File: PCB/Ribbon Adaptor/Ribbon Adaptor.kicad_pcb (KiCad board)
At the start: 2 copper layers, 20 x 24.5 mm, 6 parts, among them J1 10056847-101LF, J2 AFC07-S20FCC-00

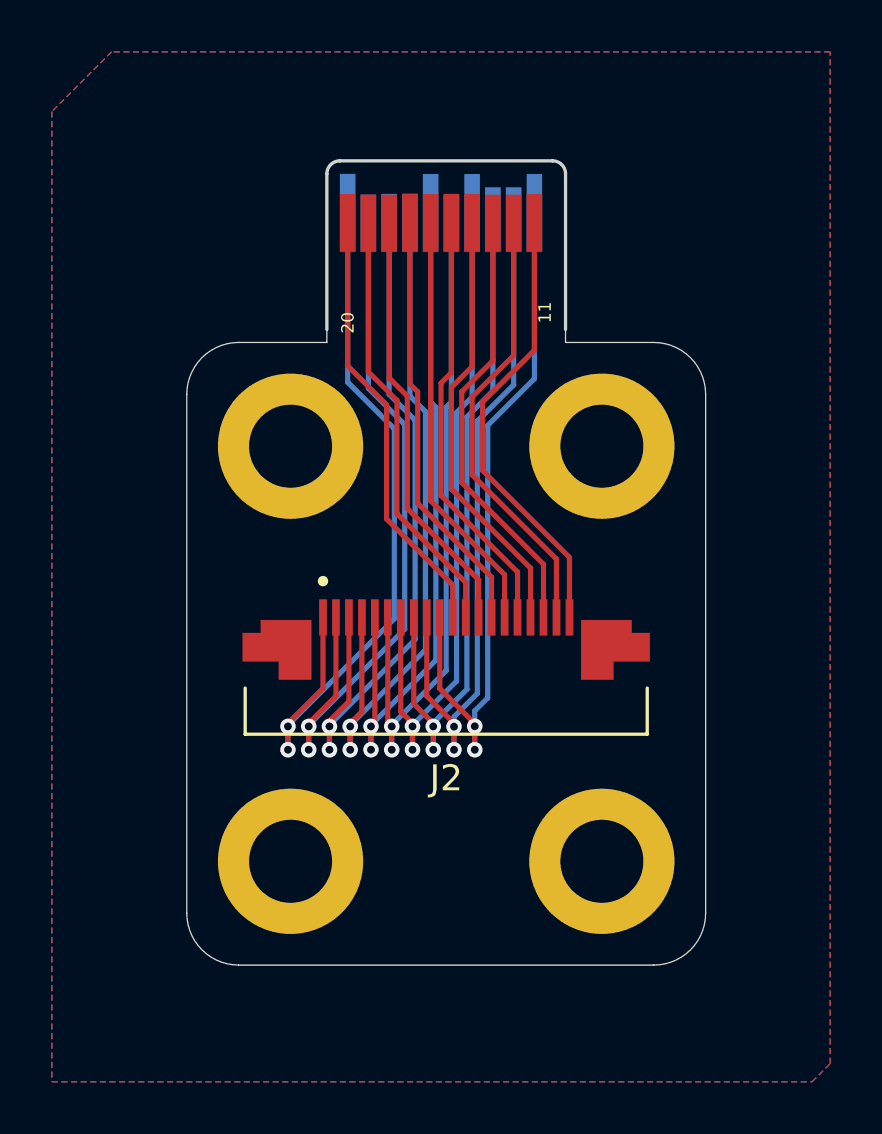
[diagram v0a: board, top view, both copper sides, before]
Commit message: Started code, commiting before adding submodules
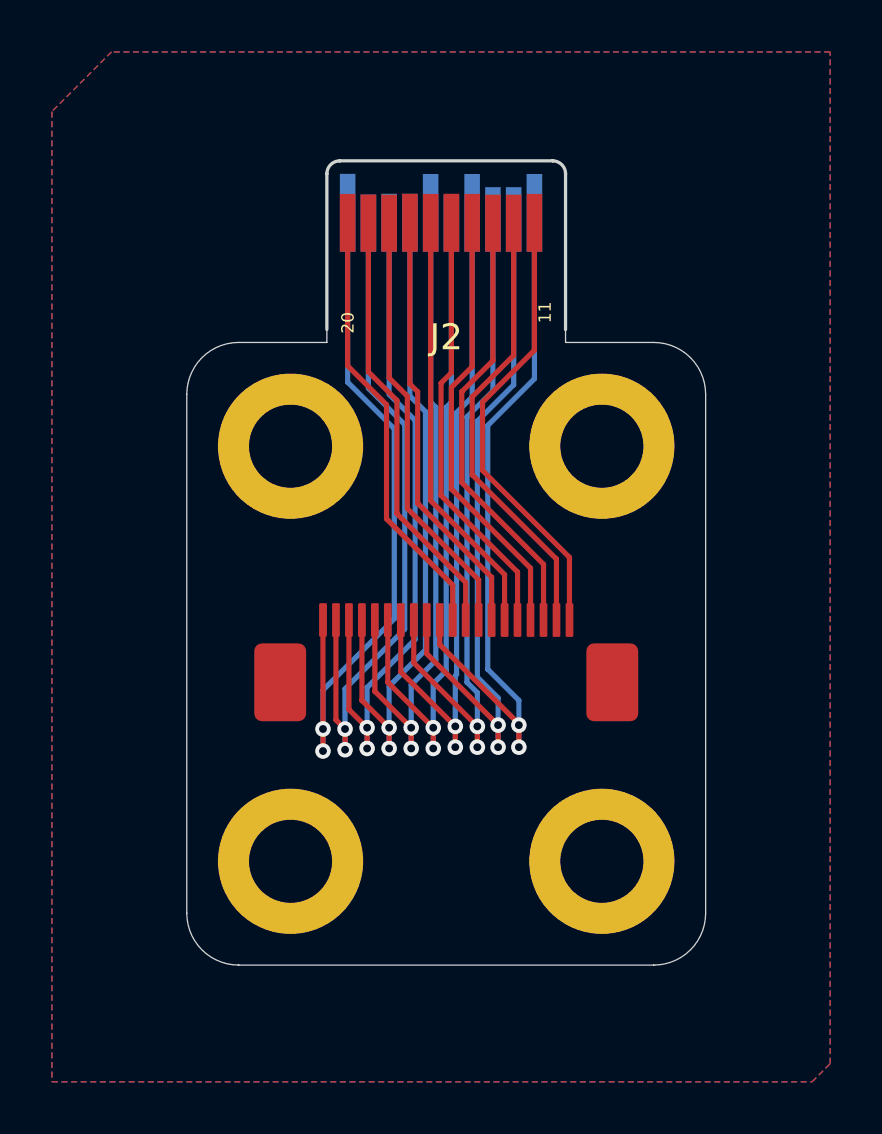
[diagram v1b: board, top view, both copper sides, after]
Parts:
- J2: footprint Snapeda:AMPHENOL_SFV20R-2STE1HLF -> Snapeda:JUSHUO AFC07-S20FCC-00
- moved J2 2.30 mm to (125.0, 59.7)
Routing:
- net /1: track 28.8 -> 27.7 mm
- net /2: track 27.9 -> 27.0 mm
- net /3: track 27.5 -> 26.7 mm
- net /10: track 27.3 -> 28.0 mm
- net /4: track 27.1 -> 26.5 mm
